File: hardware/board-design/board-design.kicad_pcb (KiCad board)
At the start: 4 copper layers, 19 parts, among them J1 Conn_01x02_Pin, U1 LM25139

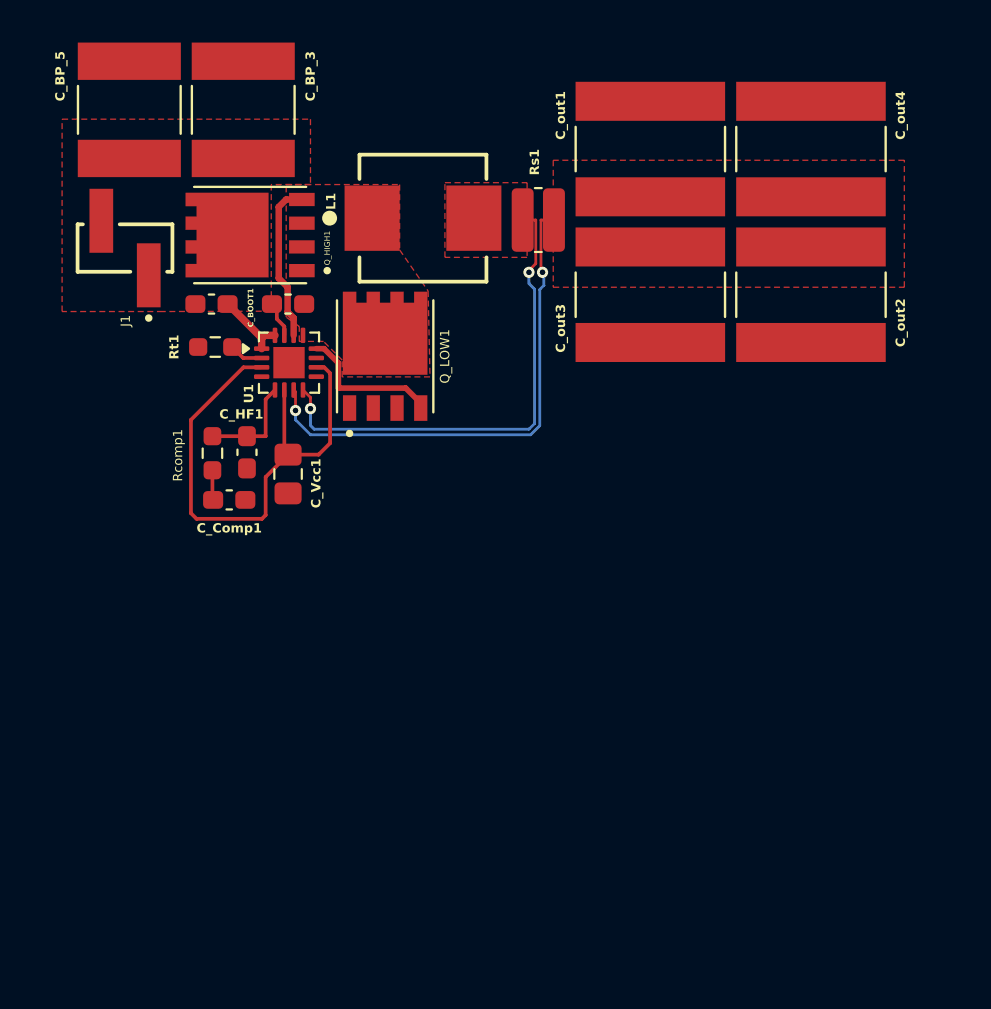
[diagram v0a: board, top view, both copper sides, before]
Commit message: feat(pcb): complate the pcb design
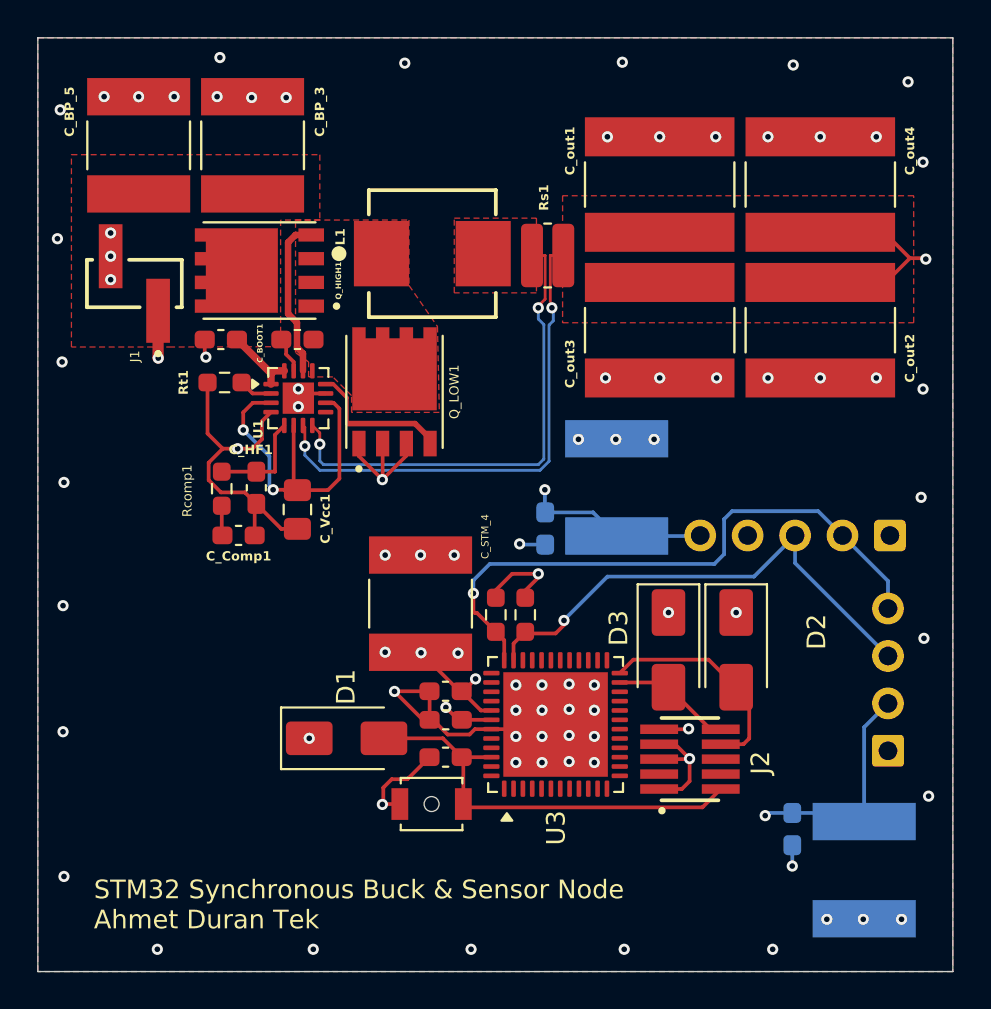
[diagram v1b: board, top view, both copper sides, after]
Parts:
- added C_STM_1: 0.1uF, Capacitor_SMD:C_0603_1608Metric_Pad1.08x0.95mm_HandSolder, F.Cu at (146.4, 118.4)
- added C_STM_2: 0.1uF, Capacitor_SMD:C_0603_1608Metric_Pad1.08x0.95mm_HandSolder, F.Cu at (146.4, 120.4)
- added C_STM_3: 0.1uF, Capacitor_SMD:C_0603_1608Metric_Pad1.08x0.95mm_HandSolder, F.Cu at (146.4, 116.8)
- added C_STM_4: 10uF, Custom-lib:CAPC6153X390N, F.Cu at (145.1, 112.1)
- added C_STM_5: 10uF, Custom-lib:CAPC6153X390N, B.Cu at (168.8, 126.4)
- added C_STM_6: 0.1uF, Capacitor_SMD:C_0603_1608Metric_Pad1.08x0.95mm_HandSolder, B.Cu at (165.0, 124.2)
- added C_STM_7: 10uF, Custom-lib:CAPC6153X390N, B.Cu at (155.6, 105.9)
- added C_STM_8: 0.1uF, Capacitor_SMD:C_0603_1608Metric_Pad1.08x0.95mm_HandSolder, B.Cu at (151.8, 108.1)
- added D1: D_TVS, Diode_SMD:D_SMA, F.Cu at (141.1, 119.4)
- added D2: D_TVS, Diode_SMD:D_SMA, F.Cu at (162.0, 114.6)
- added D3: D_TVS, Diode_SMD:D_SMA, F.Cu at (158.4, 114.6)
- added J2: Conn_02x05_Odd_Even, Custom-lib:SAMTEC_FTE-105-01-G-DV, F.Cu at (159.5, 120.5)
- added R_OpenDrain1: 4.7k, Resistor_SMD:R_0603_1608Metric_Pad0.98x0.95mm_HandSolder, F.Cu at (149.1, 112.7)
- added R_OpenDrain2: 4.7k, Resistor_SMD:R_0603_1608Metric_Pad0.98x0.95mm_HandSolder, F.Cu at (150.7, 112.7)
- added SW1: SW_Push, Button_Switch_SMD:SW_SPST_B3U-1000P-B, F.Cu at (145.7, 122.9)
- added U2: ER_OLEDM0.91_1x-I2C, Display:ER_OLEDM0.91_1x-I2C, B.Cu at (170.1, 120.0)
- added U3: STM32C031C6Ux, Package_DFN_QFN:QFN-48-1EP_7x7mm_P0.5mm_EP5.6x5.6mm, F.Cu at (152.3, 118.6)
- added U4: BMP180, Custom-lib:GY-68, B.Cu at (165.3, 92.7)
- moved C_BOOT1 1.96 mm to (138.5, 98.0)
- moved C_BP_4 1.96 mm to (134.4, 98.0)
- moved C_HF1 1.96 mm to (136.3, 105.9)
- moved C_out1 1.96 mm to (157.9, 89.7)
- moved C_out2 1.96 mm to (166.5, 97.5)
- moved C_out3 1.96 mm to (157.9, 97.5)
- moved C_out4 1.96 mm to (166.5, 89.7)
- moved J1 1.96 mm to (129.8, 95.0)
- moved L1 1.96 mm to (145.7, 93.4)
- moved Q_HIGH1 1.96 mm to (136.5, 94.3)
- moved Rs1 1.96 mm to (151.9, 93.5)
- moved U1 1.96 mm to (138.6, 101.1)
- moved C_BP_3 1.96 mm to (136.1, 87.6)
- moved C_BP_5 1.96 mm to (130.0, 87.6)
- moved C_Comp1 1.96 mm to (135.3, 108.5)
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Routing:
- net GND: track 0.00 -> 54.1 mm, vias 0 -> 81
- net /DC-DC-Buck-Converter/V_OUT: track 27.5 -> 76.4 mm, vias 2 -> 12
- net Net-(U2-SDA): track 0.00 -> 32.9 mm, vias 0 -> 1
- net Net-(U2-SCL): track 0.00 -> 27.1 mm, vias 0 -> 1
- net /STM32/NRST: track 0.00 -> 22.9 mm
- net Net-(D2-A2): track 0.00 -> 11.8 mm
- net /DC-DC-Buck-Converter/Vcc: track 28.6 -> 18.5 mm, vias 0 -> 2
- net Net-(D3-A2): track 0.00 -> 6.45 mm
- net /DC-DC-Buck-Converter/V_INPUT: track 4.21 -> 6.74 mm, vias 0 -> 1
- added copper zone on In2.Cu, net /DC-DC-Buck-Converter/V_INPUT
- added copper zone on In2.Cu, net /DC-DC-Buck-Converter/V_OUT
- added copper zone on B.Cu, net GND
- added copper zone on F.Cu, net GND
- added copper zone on In1.Cu, net GND
- added copper zone on In2.Cu, net GND
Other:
- board outline added: 49 x 50 mm
- board text added: "STM32 Synchronous Buck & Sensor Node Ahmet Duran Tek"
